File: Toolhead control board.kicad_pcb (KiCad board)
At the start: 2 copper layers, 51.6 x 31.4 mm, 53 parts, among them J1 Conn_01x02_Pin, J12 Conn_01x04_Male, J2 Conn_01x02_Pin, J3 Conn_01x06_Pin, J4 Conn_01x02_Pin, J5 Conn_01x02_Pin, J6 Conn_01x02_Pin, J7 USB_C_Receptacle_USB2.0_14P, Q1 AS3400, Q2 AS3400, Q3 AS3400, U1 ADXL345, U2 STM32F042G6Ux, U3 TMC2209, U4 AP63205WU, U5 MCP1802x-xx02xOT, Y1 8MHz

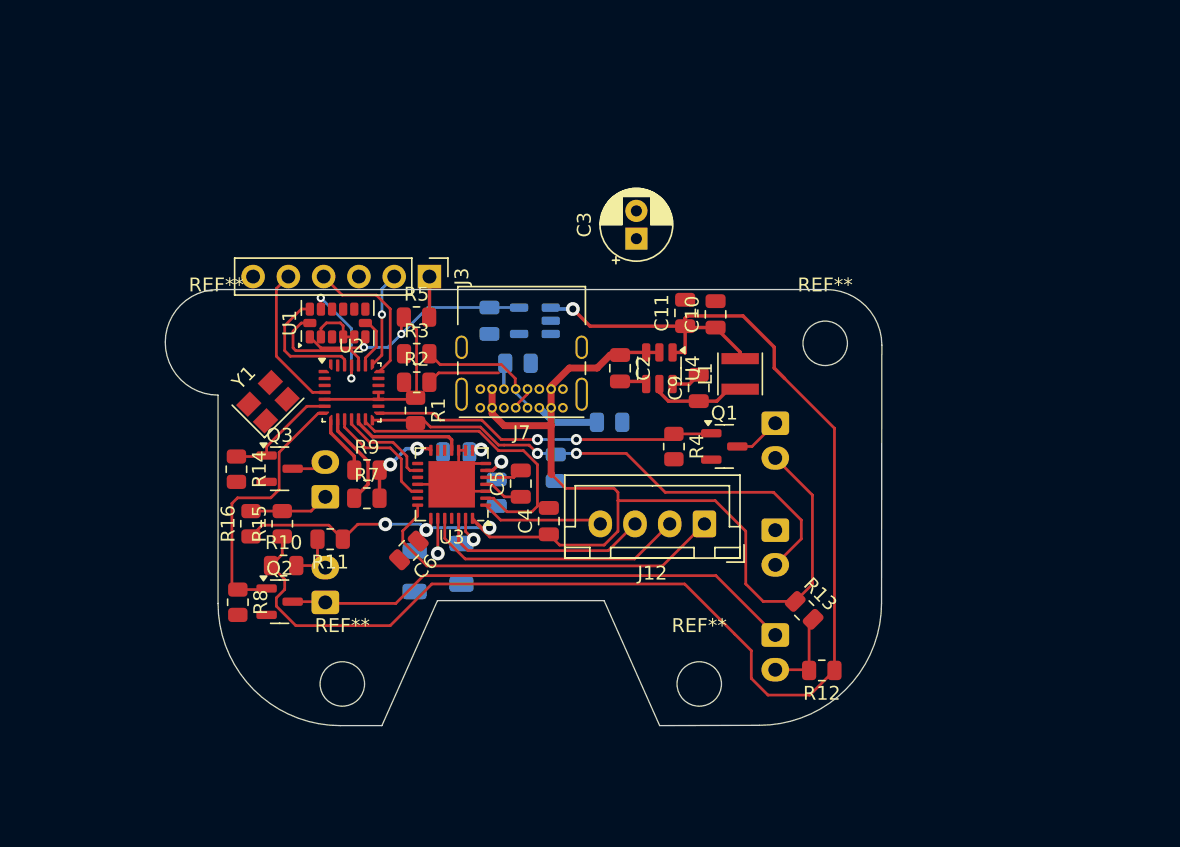
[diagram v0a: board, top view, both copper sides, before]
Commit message: Rev1. Uart interface
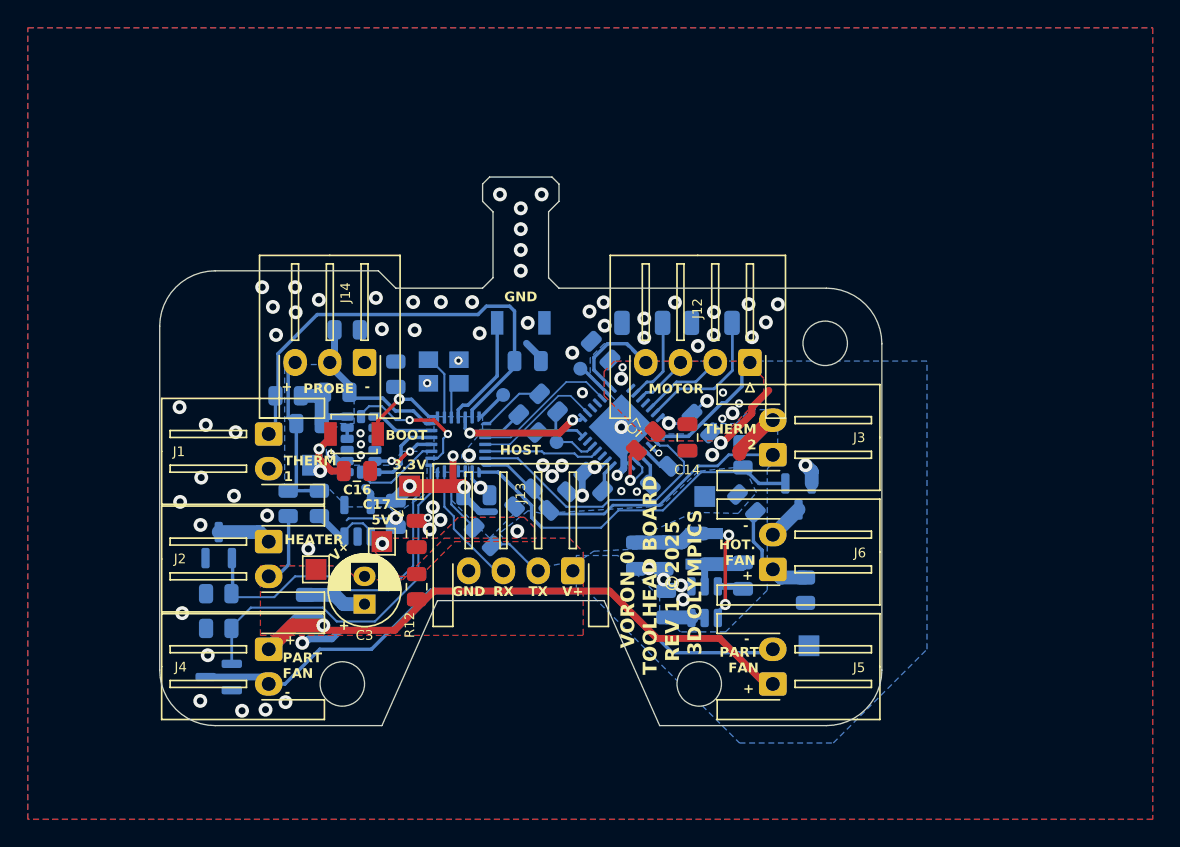
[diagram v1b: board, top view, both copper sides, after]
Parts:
- removed J7: USB_C_Receptacle_USB2.0_14P, Connector_USB:USB_C_Receptacle_GCT_USB4085
- removed R10, R11, R5: OPEN, Resistor_SMD:R_0805_2012Metric
- removed R17, R20: 5.1k, Resistor_SMD:R_0805_2012Metric
- added C13: C, Capacitor_SMD:C_0805_2012Metric, B.Cu at (152.7, 86.8)
- added C14: 10uF, Capacitor_SMD:C_0805_2012Metric, F.Cu at (162.0, 82.2)
- added C15: 1uF, Capacitor_SMD:C_0805_2012Metric, B.Cu at (146.8, 86.4)
- added C16: 1uF, Capacitor_SMD:C_0805_2012Metric, F.Cu at (138.2, 84.7)
- added C17: 4.7uF, Capacitor_SMD:C_0805_2012Metric, F.Cu at (142.5, 89.2)
- added J13: Conn_01x04_Male, Connector_JST:JST_XH_S4B-XH-A-1_1x04_P2.50mm_Horizontal, F.Cu at (153.8, 91.8)
- added J14: Conn_01x04_Male, Connector_JST:JST_XH_S3B-XH-A-1_1x03_P2.50mm_Horizontal, F.Cu at (138.8, 76.8)
- added R21: OPEN, Resistor_SMD:R_0805_2012Metric, B.Cu at (135.5, 87.0)
- added R22: OPEN, Resistor_SMD:R_0805_2012Metric, B.Cu at (133.2, 87.0)
- added R23: OPEN, Resistor_SMD:R_0805_2012Metric, B.Cu at (134.8, 81.2)
- added R24: OPEN, Resistor_SMD:R_0805_2012Metric, B.Cu at (136.8, 79.0)
- added R25: OPEN, Resistor_SMD:R_0805_2012Metric, B.Cu at (137.5, 74.5)
- added R6: 22k, Resistor_SMD:R_0805_2012Metric, B.Cu at (141.0, 77.7)
- added REF**: TestPoint_Pad_1.5x1.5mm, TestPoint:TestPoint_Pad_1.5x1.5mm, F.Cu at (140.0, 89.8)
- added REF**: TestPoint_Pad_1.5x1.5mm, TestPoint:TestPoint_Pad_1.5x1.5mm, B.Cu at (135.0, 84.2)
- added REF**: TestPoint_Pad_1.5x1.5mm, TestPoint:TestPoint_Pad_1.5x1.5mm, F.Cu at (142.0, 85.8)
- added REF**: TestPoint_Pad_1.5x1.5mm, TestPoint:TestPoint_Pad_1.5x1.5mm, F.Cu at (135.2, 91.8)
- added REF**: TestPoint_Pad_1.5x1.5mm, TestPoint:TestPoint_Pad_1.5x1.5mm, B.Cu at (163.2, 86.5)
- added REF**: TestPoint_Pad_1.5x1.5mm, TestPoint:TestPoint_Pad_1.5x1.5mm, B.Cu at (170.8, 97.2)
- added SW1: SW_SPST, Button_Switch_SMD:SW_SPST_B3U-1000P, B.Cu at (150.0, 74.0)
- added SW2: SW_SPST, Button_Switch_SMD:SW_SPST_B3U-1000P, F.Cu at (138.0, 82.0)
- added TP1: TestPoint_Probe, TestPoint:TestPoint_Pad_D1.0mm, B.Cu at (152.6, 82.6)
- added TP2: TestPoint_Probe, TestPoint:TestPoint_Pad_D1.0mm, B.Cu at (154.3, 77.3)
- added TP3: TestPoint_Probe, TestPoint:TestPoint_Pad_D1.0mm, B.Cu at (148.7, 79.2)
- C10, C11, C2, C4, C5, C6, C9, L1, Q1, Q2, Q3, R1, R13, R14, R15, R16, R2, R4, R7, R8, R9, U1, U2, U3, U4, Y1: moved to B.Cu
- C7, J1, J2, J4, J5, J6: moved to F.Cu
- J12: footprint Connector_JST:JST_XH_B4B-XH-A_1x04_P2.50mm_Vertical -> Connector_JST:JST_XH_S4B-XH-A-1_1x04_P2.50mm_Horizontal
- J3: value Conn_01x06_Pin -> Conn_01x02_Pin; footprint Connector_PinHeader_2.54mm:PinHeader_1x06_P2.54mm_Vertical -> Connector_JST:JST_XH_S2B-XH-A-1_1x02_P2.50mm_Horizontal
- R3: value 27 -> 4.7k; moved to B.Cu
- moved R16 40.2 mm to (170.5, 93.2)
- moved J2 37.5 mm to (131.8, 89.8)
- moved Q3 37.4 mm to (170.0, 86.5), turned to -90 degrees
- moved J1 37.1 mm to (131.8, 82.0)
- moved Q1 37.1 mm to (128.2, 90.0), turned to 90 degrees
- moved R14 36.5 mm to (166.0, 83.5), turned to 90 degrees
- moved R13 35.9 mm to (134.5, 94.5), turned to -90 degrees
- moved R4 34.4 mm to (128.2, 93.5), turned to 180 degrees
- moved R15 33.5 mm to (166.2, 87.0), turned to -45 degrees
- moved C3 32.8 mm to (138.8, 94.2)
- moved J6 32.6 mm to (168.2, 91.8)
- moved R12 29.8 mm to (142.5, 93.0), turned to -90 degrees
- moved J3 27.9 mm to (168.2, 83.5), turned to 90 degrees
- moved R18 25.0 mm to (163.8, 74.0), turned to 180 degrees
- moved R19 24.3 mm to (158.8, 74.0), turned to 180 degrees
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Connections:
- C1 pad 1: THERMISTOR -> THERMISTOR_1
- J1 pad 1: GND -> THERMISTOR_1
- J1 pad 2: THERMISTOR -> GND
- J3 pad 1: Net-(J3-Pin_1) -> THERMISTOR_2
- J3 pad 2: Net-(J3-Pin_2) -> GND
- J5 pad 2: Net-(J5-Pin_2) -> Net-(J4-Pin_2)
- Q2 pad 3: Net-(J4-Pin_1) -> Net-(J4-Pin_2)
- R1 pad 2: THERMISTOR -> THERMISTOR_1
- R12 pad 2: Net-(J5-Pin_2) -> Net-(J4-Pin_1)
- R13 pad 2: Net-(J5-Pin_2) -> Net-(J4-Pin_1)
- R2 pad 2: D- -> TX
- R3 pad 1: Net-(U2-PA10/PA12) -> +3.3V
- R3 pad 2: D+ -> THERMISTOR_2
- U1 pad 8: unconnected-(U1-INT1-Pad8) -> ADXL_INT
- U2 pad 1: unconnected-(U2-PB8-Pad1) -> Net-(SW2-B)
- U2 pad 14: THERMISTOR -> THERMISTOR_2
- U2 pad 15: HEATER -> HOTEND_FAN
- U2 pad 20: Net-(U2-PA10/PA12) -> RX
- U2 pad 21: Net-(J3-Pin_4) -> PART_FAN
- U2 pad 22: Net-(J3-Pin_2) -> HEATER
- U2 pad 27: unconnected-(U2-PB6-Pad27) -> ADXL_INT
- U2 pad 28: unconnected-(U2-PB7-Pad28) -> PROBE
- U2 pad 4: NRST -> Net-(SW1-B)
- U2 pad 6: HOTEND_FAN -> THERMISTOR_1
- U2 pad 7: PART_FAN -> Net-(U2-PA1)
- U3 pad 1: Net-(J12-Pin_4) -> Net-(J12-Pin_1)
- U3 pad 15: +3V3 -> +3.3V
- U3 pad 21: Net-(J12-Pin_1) -> Net-(J12-Pin_4)
- U3 pad 24: Net-(J12-Pin_2) -> Net-(J12-Pin_3)
- U3 pad 26: Net-(J12-Pin_3) -> Net-(J12-Pin_2)
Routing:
- net +5V: track 104.6 -> 19.9 mm, vias 1 -> 4
- net +VDC: track 92.4 -> 17.0 mm, vias 3 -> 8
- net Net-(J4-Pin_2): track 4.43 -> 45.8 mm
- net THERMISTOR: track 37.9 -> 0.00 mm, vias 2 -> 0
- net THERMISTOR_1: track 0.00 -> 33.6 mm
- net THERMISTOR_2: track 0.00 -> 24.0 mm
- net GND: track 17.4 -> 36.7 mm, vias 0 -> 81
- net HOTEND_FAN: track 8.23 -> 26.5 mm
- net Net-(J12-Pin_1): track 26.8 -> 10.6 mm
- net Net-(J12-Pin_2): track 19.3 -> 6.23 mm
- net PROBE: track 0.00 -> 12.0 mm
- net Net-(J14-Pin_3): track 0.00 -> 11.8 mm
- net Net-(J12-Pin_3): track 16.3 -> 5.31 mm
- net NRST: track 10.6 -> 0.00 mm
- net Net-(J3-Pin_4): track 10.6 -> 0.00 mm
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- added copper zone on B.Cu, net +3.3V
- added copper zone on B.Cu, net +5V
- added copper zone on F.Cu, net +5V
- added copper zone on B.Cu, net +VDC
- added copper zone on F.Cu, net +VDC
- added copper zone on B.Cu, net GND
- added copper zone on F.Cu, net GND
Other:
- board size 51.6 x 31.4 mm -> 52 x 39.5 mm
- board text added: "+"
- board text added: "-"
- board text added: "3.3V"
- board text added: "5V"
- board text added: "BOOT"
- board text added: "GND"
- board text added: "HEATER"
- board text added: "HOST"
- board text added: "HOT- FAN END"
- board text added: "HOT. FAN"
- board text added: "HOTEND FAN"
- board text added: "MOTOR"
- board text added: "P. FAN"
- board text added: "PART FAN"
- board text added: "PROBE"
- board text added: "RESET"
- board text added: "RX"
- board text added: "THERM 1"
- board text added: "THERM 2"
- board text added: "THERMISTOR 1"
- board text added: "THERMISTOR 2"
- board text added: "TX"
- board text added: "V+"
- board text added: "VORON 0 TOOLHEAD BOARD REV 1 ©2025 3D OLYMPICS"
- board text added: "X"
- board text added: "Y"
- board text added: "Z"
